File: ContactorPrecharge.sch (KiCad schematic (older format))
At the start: 9 parts

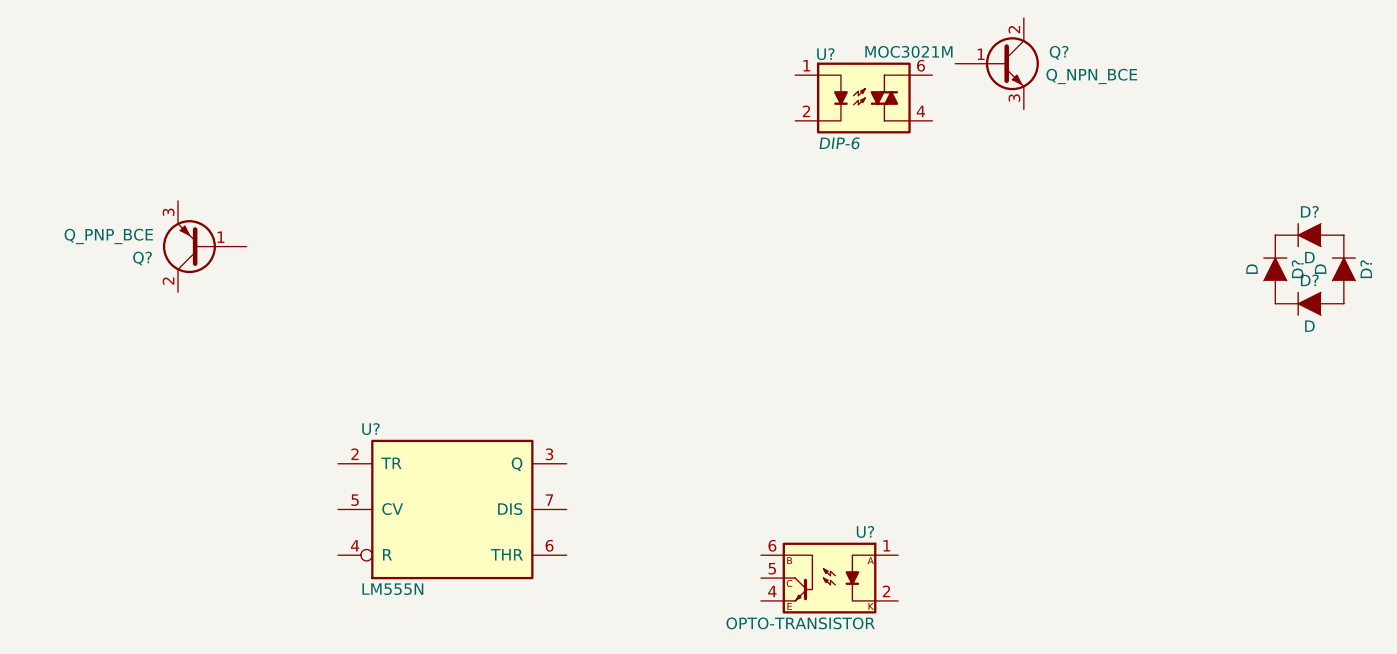
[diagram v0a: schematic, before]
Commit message: basic connectivity
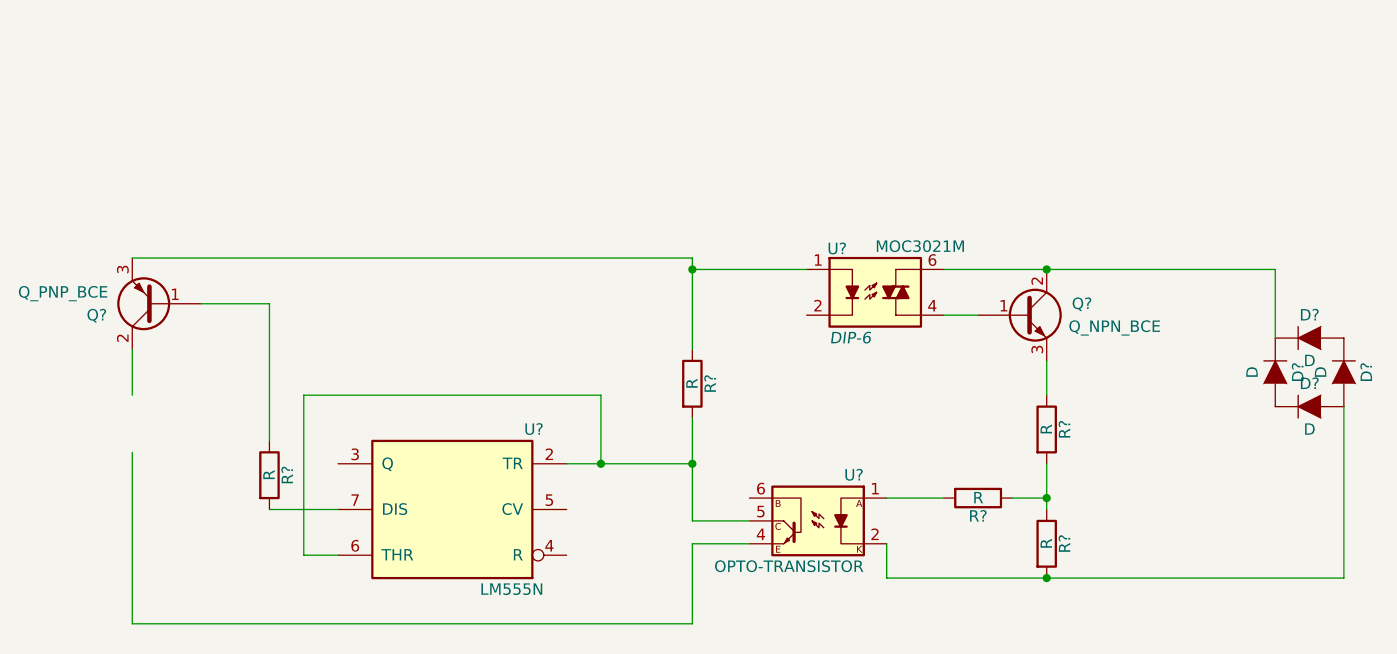
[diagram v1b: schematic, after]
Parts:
- added R? (x5): R, symbol R
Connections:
- wire segments 0 -> 28
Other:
- moved on the sheet: D?, Q?, U?
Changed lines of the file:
@@
 LIBS:contrib
 LIBS:valves
+LIBS:ContactorPrecharge-cache
 EELAYER 25 0
 EELAYER END
@@
 F 3 "" H 6250 5000 50  0000 C CNN
 	1    6250 5000
-	1    0    0    -1
+	-1   0    0    -1
 $EndComp
 $Comp
 L OPTO-TRANSISTOR U?
 U 1 1 56F0DEFB
-P 7900 5300
-F 0 "U?" H 7700 5500 50  0000 L CNN
-F 1 "OPTO-TRANSISTOR" H 7700 5100 50  0000 L CNN
-F 2 "" H 7700 5100 50  0000 L CIN
-F 3 "" H 7900 5300 50  0000 L CNN
-	1    7900 5300
+P 7850 5050
+F 0 "U?" H 7650 5250 50  0000 L CNN
+F 1 "OPTO-TRANSISTOR" H 7650 4850 50  0000 L CNN
+F 2 "" H 7650 4850 50  0000 L CIN
+F 3 "" H 7850 5050 50  0000 L CNN
+	1    7850 5050
 	-1   0    0    -1
 $EndComp
@@
 L MOC3021M U?
 U 1 1 56F0DF72
-P 8050 3200
-F 0 "U?" H 7840 3390 50  0000 L CNN
-F 1 "MOC3021M" H 8050 3400 50  0000 L CNN
-F 2 "DIP-6" H 7850 3000 50  0000 L CIN
-F 3 "" H 8025 3200 50  0000 L CNN
-	1    8050 3200
+P 8100 4050
+F 0 "U?" H 7890 4240 50  0000 L CNN
+F 1 "MOC3021M" H 8100 4250 50  0000 L CNN
+F 2 "DIP-6" H 7900 3850 50  0000 L CIN
+F 3 "" H 8075 4050 50  0000 L CNN
+	1    8100 4050
 	1    0    0    -1
 $EndComp
@@
 L Q_PNP_BCE Q?
 U 1 1 56F0E04D
-P 5150 3850
-F 0 "Q?" H 5450 3900 50  0000 R CNN
-F 1 "Q_PNP_BCE" H 5750 3800 50  0000 R CNN
-F 2 "" H 5350 3950 50  0000 C CNN
-F 3 "" H 5150 3850 50  0000 C CNN
-	1    5150 3850
+P 4950 4100
+F 0 "Q?" H 5250 4150 50  0000 R CNN
+F 1 "Q_PNP_BCE" H 5550 4050 50  0000 R CNN
+F 2 "" H 5150 4200 50  0000 C CNN
+F 3 "" H 4950 4100 50  0000 C CNN
+	1    4950 4100
 	-1   0    0    1
 $EndComp
@@
 L Q_NPN_BCE Q?
 U 1 1 56F0E0BE
-P 8650 3050
-F 0 "Q?" H 8950 3100 50  0000 R CNN
-F 1 "Q_NPN_BCE" H 9250 3000 50  0000 R CNN
-F 2 "" H 8850 3150 50  0000 C CNN
-F 3 "" H 8650 3050 50  0000 C CNN
-	1    8650 3050
+P 8750 4150
+F 0 "Q?" H 9050 4200 50  0000 R CNN
+F 1 "Q_NPN_BCE" H 9350 4100 50  0000 R CNN
+F 2 "" H 8950 4250 50  0000 C CNN
+F 3 "" H 8750 4150 50  0000 C CNN
+	1    8750 4150
 	1    0    0    -1
 $EndComp
@@
 L D D?
 U 1 1 56F0E506
-P 10000 3800
-F 0 "D?" H 10000 3900 50  0000 C CNN
-F 1 "D" H 10000 3700 50  0000 C CNN
-F 2 "" H 10000 3800 50  0000 C CNN
-F 3 "" H 10000 3800 50  0000 C CNN
-	1    10000 3800
+P 10000 4250
+F 0 "D?" H 10000 4350 50  0000 C CNN
+F 1 "D" H 10000 4150 50  0000 C CNN
+F 2 "" H 10000 4250 50  0000 C CNN
+F 3 "" H 10000 4250 50  0000 C CNN
+	1    10000 4250
 	1    0    0    -1
 $EndComp
@@
 L D D?
 U 1 1 56F0E5AD
-P 9850 3950
-F 0 "D?" H 9850 4050 50  0000 C CNN
-F 1 "D" H 9850 3850 50  0000 C CNN
-F 2 "" H 9850 3950 50  0000 C CNN
-F 3 "" H 9850 3950 50  0000 C CNN
-	1    9850 3950
+P 9850 4400
+F 0 "D?" H 9850 4500 50  0000 C CNN
+F 1 "D" H 9850 4300 50  0000 C CNN
+F 2 "" H 9850 4400 50  0000 C CNN
+F 3 "" H 9850 4400 50  0000 C CNN
+	1    9850 4400
 	0    1    1    0
 $EndComp
@@
 L D D?
 U 1 1 56F0E5FE
-P 10000 4100
-F 0 "D?" H 10000 4200 50  0000 C CNN
-F 1 "D" H 10000 4000 50  0000 C CNN
-F 2 "" H 10000 4100 50  0000 C CNN
-F 3 "" H 10000 4100 50  0000 C CNN
-	1    10000 4100
+P 10000 4550
+F 0 "D?" H 10000 4650 50  0000 C CNN
+F 1 "D" H 10000 4450 50  0000 C CNN
+F 2 "" H 10000 4550 50  0000 C CNN
+F 3 "" H 10000 4550 50  0000 C CNN
+	1    10000 4550
 	1    0    0    -1
 $EndComp
@@
 L D D?
 U 1 1 56F0E64E
-P 10150 3950
-F 0 "D?" H 10150 4050 50  0000 C CNN
-F 1 "D" H 10150 3850 50  0000 C CNN
-F 2 "" H 10150 3950 50  0000 C CNN
-F 3 "" H 10150 3950 50  0000 C CNN
-	1    10150 3950
+P 10150 4400
+F 0 "D?" H 10150 4500 50  0000 C CNN
+F 1 "D" H 10150 4300 50  0000 C CNN
+F 2 "" H 10150 4400 50  0000 C CNN
+F 3 "" H 10150 4400 50  0000 C CNN
+	1    10150 4400
 	0    1    1    0
 $EndComp
+$Comp
+L R R?
+U 1 1 56F0F035
+P 5450 4850
+F 0 "R?" V 5530 4850 50  0000 C CNN
+F 1 "R" V 5450 4850 50  0000 C CNN
+F 2 "" V 5380 4850 50  0000 C CNN
+F 3 "" H 5450 4850 50  0000 C CNN
+	1    5450 4850
+	1    0    0    -1
+$EndComp
+Wire Wire Line
+	5450 5000 5750 5000
+Wire Wire Line
+	5150 4100 5450 4100
+Wire Wire Line
+	5450 4100 5450 4700
+Wire Wire Line
+	5750 5200 5600 5200
+Wire Wire Line
+	5600 5200 5600 4500
+Wire Wire Line
+	5600 4500 6900 4500
+Wire Wire Line
+	6900 4500 6900 4800
+Wire Wire Line
+	6750 4800 7300 4800
+Wire Wire Line
+	7300 5050 7550 5050
+Wire Wire Line
+	7300 4600 7300 5050
+Connection ~ 6900 4800
+$Comp
+L R R?
+U 1 1 56F0F2E6
+P 7300 4450
+F 0 "R?" V 7380 4450 50  0000 C CNN
+F 1 "R" V 7300 4450 50  0000 C CNN
+F 2 "" V 7230 4450 50  0000 C CNN
+F 3 "" H 7300 4450 50  0000 C CNN
+	1    7300 4450
+	1    0    0    -1
+$EndComp
+Connection ~ 7300 4800
+Wire Wire Line
+	7300 4300 7300 3900
+Wire Wire Line
+	7300 3900 4850 3900
+$Comp
+L R R?
+U 1 1 56F0F46B
+P 8850 4650
+F 0 "R?" V 8930 4650 50  0000 C CNN
+F 1 "R" V 8850 4650 50  0000 C CNN
+F 2 "" V 8780 4650 50  0000 C CNN
+F 3 "" H 8850 4650 50  0000 C CNN
+	1    8850 4650
+	1    0    0    -1
+$EndComp
+$Comp
+L R R?
+U 1 1 56F0F4DF
+P 8850 5150
+F 0 "R?" V 8930 5150 50  0000 C CNN
+F 1 "R" V 8850 5150 50  0000 C CNN
+F 2 "" V 8780 5150 50  0000 C CNN
+F 3 "" H 8850 5150 50  0000 C CNN
+	1    8850 5150
+	1    0    0    -1
+$EndComp
+Wire Wire Line
+	8400 3950 9850 3950
+Wire Wire Line
+	8550 4150 8400 4150
+Wire Wire Line
+	8850 4500 8850 4350
+Wire Wire Line
+	8850 5000 8850 4800
+$Comp
+L R R?
+U 1 1 56F0F6F1
+P 8550 4950
+F 0 "R?" V 8630 4950 50  0000 C CNN
+F 1 "R" V 8550 4950 50  0000 C CNN
+F 2 "" V 8480 4950 50  0000 C CNN
+F 3 "" H 8550 4950 50  0000 C CNN
+	1    8550 4950
+	0    1    1    0
+$EndComp
+Wire Wire Line
+	8700 4950 8850 4950
+Connection ~ 8850 4950
+Wire Wire Line
+	9850 3950 9850 4250
+Connection ~ 8850 3950
+Wire Wire Line
+	10150 5300 10150 4550
+Wire Wire Line
+	8150 5300 10150 5300
+Wire Wire Line
+	8150 5150 8150 5300
+Connection ~ 8850 5300
+Wire Wire Line
+	8400 4950 8150 4950
+Wire Wire Line
+	7550 5150 7300 5150
+Wire Wire Line
+	7300 5150 7300 5500
+Wire Wire Line
+	7300 5500 4850 5500
+Wire Wire Line
+	4850 5500 4850 4750
+Wire Wire Line
+	4850 4300 4850 4500
+Wire Wire Line
+	7800 3950 7300 3950
+Connection ~ 7300 3950
 $EndSCHEMATC
